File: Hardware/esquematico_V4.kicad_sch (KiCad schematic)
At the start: 7 parts, among them J11 Conn_01x02_Socket, J4 Conn_cartao_SD, J5 Conn_BH1750, J6 Conn_BMP, U2 module_bh1750, U3 module_bme280, U6 MicroSD Card Adapter

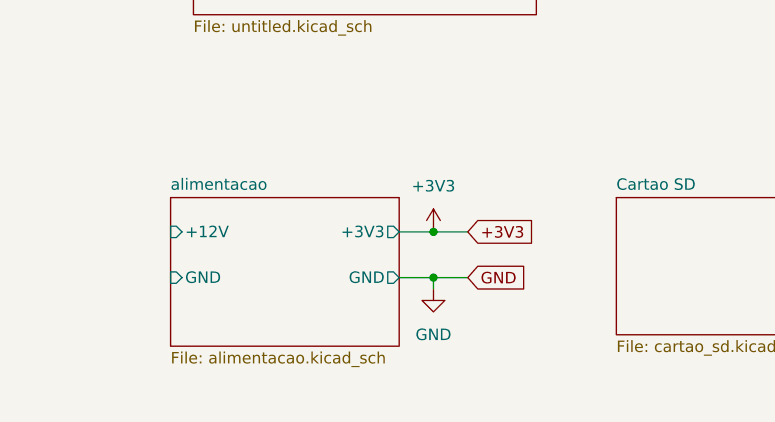
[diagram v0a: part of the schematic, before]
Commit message: hardware: implementa alimentacao e adiciona bibliotecas locais - ajuda gpt
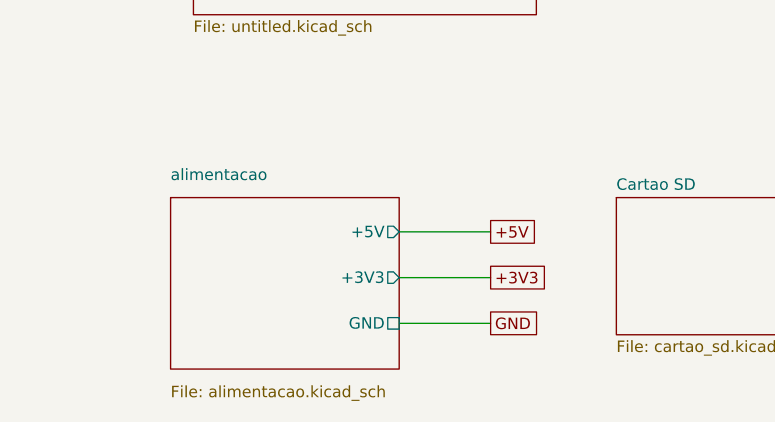
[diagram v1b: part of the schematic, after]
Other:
- sheet alimentacao ports: added +5V; removed +12V
